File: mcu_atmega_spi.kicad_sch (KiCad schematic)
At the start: 34 parts, among them J10 Conn_01x01, J5 AVR ICSP, J6 Conn_01x01, J7 Conn_01x01, J8 Conn_01x01, J9 Conn_01x01, SW1 SW_Push, SW2 SW_Push, SW3 SW_Push, U5 ATmega328P-A, U6 CP2102N-A02-GQFN28, Y2 Crystal_GND24

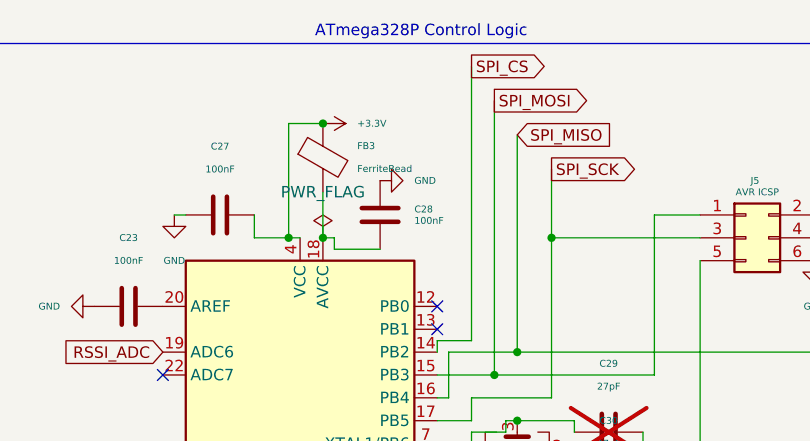
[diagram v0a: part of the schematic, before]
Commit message: done with lcsc
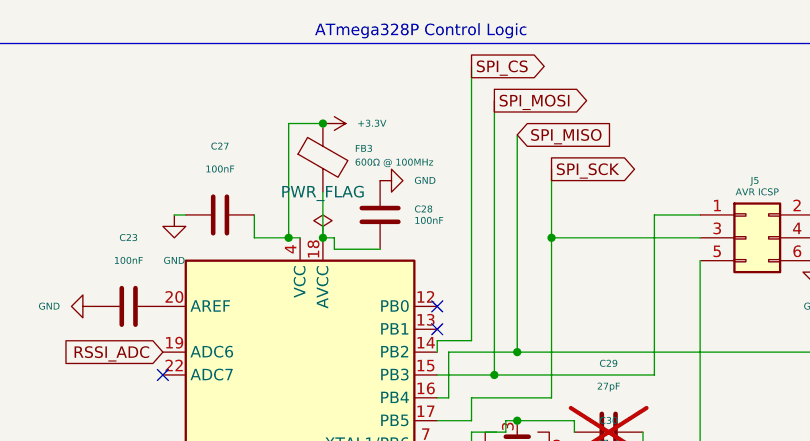
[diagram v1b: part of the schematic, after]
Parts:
- C1, C2, C23, C27, C28, C3, C31, C32: LCSC C1591 -> C1711
- C29, C30: LCSC (none) -> C472840
- FB3: value FerriteBead -> 600Ω @ 100MHz; LCSC C1015 -> C21519
- J5: LCSC C65114 -> (none)
- R15: LCSC (none) -> C2933324
- R18, R19, R21, R22, R23, R3: LCSC C25744 -> C543567
- SW1, SW2, SW3: LCSC C318884 -> C2834918
- U6: LCSC C1550553 -> C964632
- Y2: LCSC C13738 -> C7275095
